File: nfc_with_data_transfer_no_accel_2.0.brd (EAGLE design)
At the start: 13.2 x 18.4 mm, 7 parts

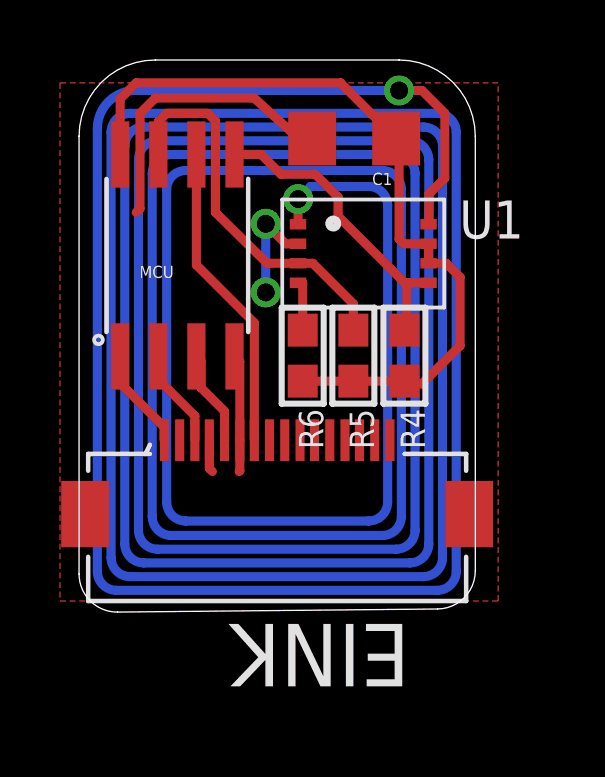
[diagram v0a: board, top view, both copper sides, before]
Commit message: fixed rst
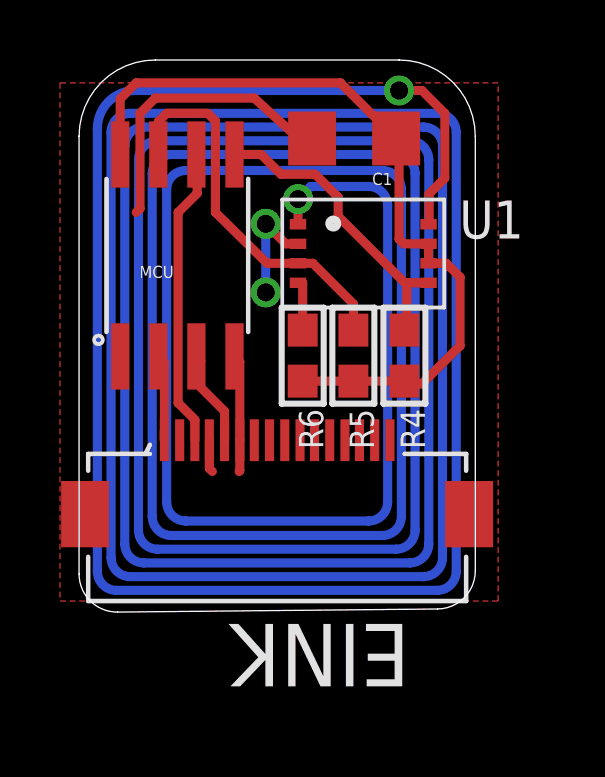
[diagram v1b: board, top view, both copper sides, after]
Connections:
- net DOT1: now also MCU.6; no longer MCU.2
- net DOT5: now also MCU.1; no longer MCU.6
- net RST: now also MCU.2; no longer MCU.1
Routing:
- net DOT5: track 10.3 -> 0.00 mm
- net DOT1: track 3.30 -> 10.0 mm
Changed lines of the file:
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@@
 <layer number="14" name="Route14" color="1" fill="6" visible="no" active="no"/>
 <layer number="15" name="Route15" color="4" fill="6" visible="no" active="no"/>
-<layer number="16" name="Bottom" color="1" fill="1" visible="yes" active="yes"/>
+<layer number="16" name="Bottom" color="1" fill="1" visible="no" active="yes"/>
 <layer number="17" name="Pads" color="2" fill="1" visible="yes" active="yes"/>
 <layer number="18" name="Vias" color="2" fill="1" visible="yes" active="yes"/>
@@
 <contactref element="EINK" pad="5"/>
 <contactref element="MCU" pad="3"/>
+<wire x1="7.5946" y1="10.4394" x2="7.747" y2="10.287" width="0.3048" layer="1"/>
 <wire x1="8.5344" y1="7.6454" x2="8.5344" y2="8.6106" width="0.3048" layer="1"/>
-<wire x1="8.5344" y1="8.6106" x2="7.747" y2="9.398" width="0.3048" layer="1"/>
-<wire x1="7.747" y1="9.398" x2="7.747" y2="10.287" width="0.3048" layer="1"/>
-<wire x1="7.747" y1="10.287" x2="7.5946" y2="10.4394" width="0.3048" layer="1"/>
+<wire x1="8.5344" y1="8.6106" x2="7.62" y2="9.525" width="0.3048" layer="1"/>
+<wire x1="7.62" y1="9.525" x2="7.62" y2="10.414" width="0.3048" layer="1"/>
+<wire x1="7.62" y1="10.414" x2="7.5946" y2="10.4394" width="0.3048" layer="1"/>
 </signal>
 <signal name="DOT1">
 <contactref element="EINK" pad="3"/>
-<contactref element="MCU" pad="2"/>
-<wire x1="7.5438" y1="7.6454" x2="7.5438" y2="8.4582" width="0.3048" layer="1"/>
-<wire x1="7.5438" y1="8.4582" x2="6.35" y2="9.652" width="0.3048" layer="1"/>
-<wire x1="6.35" y1="9.652" x2="6.35" y2="10.414" width="0.3048" layer="1"/>
-<wire x1="6.35" y1="10.414" x2="6.3246" y2="10.4394" width="0.3048" layer="1"/>
+<contactref element="MCU" pad="6"/>
+<wire x1="7.5438" y1="7.6454" x2="7.5438" y2="8.3312" width="0.3048" layer="1"/>
+<wire x1="7.5438" y1="8.3312" x2="6.985" y2="8.89" width="0.3048" layer="1"/>
+<wire x1="6.985" y1="8.89" x2="6.985" y2="15.24" width="0.3048" layer="1"/>
+<wire x1="6.985" y1="15.24" x2="7.62" y2="15.875" width="0.3048" layer="1"/>
+<wire x1="7.62" y1="15.875" x2="7.62" y2="17.145" width="0.3048" layer="1"/>
+<wire x1="7.62" y1="17.145" x2="7.5946" y2="17.1704" width="0.3048" layer="1"/>
 </signal>
 <signal name="RST">
 <contactref element="EINK" pad="1"/>
-<contactref element="MCU" pad="1"/>
 <wire x1="6.5278" y1="7.9502" x2="6.5278" y2="7.6454" width="0.3048" layer="1"/>
-<wire x1="6.5278" y1="7.6454" x2="6.5278" y2="8.0772" width="0.3048" layer="1"/>
 <wire x1="5.08" y1="9.525" x2="5.08" y2="10.414" width="0.3048" layer="1"/>
-<wire x1="5.08" y1="10.414" x2="5.0546" y2="10.4394" width="0.3048" layer="1"/>
-<wire x1="6.5278" y1="7.6454" x2="6.5278" y2="8.0772" width="0.3048" layer="1"/>
-<wire x1="6.5278" y1="8.0772" x2="5.08" y2="9.525" width="0.3048" layer="1"/>
+<contactref element="MCU" pad="2"/>
+<wire x1="6.5278" y1="7.6454" x2="6.5278" y2="10.2362" width="0.3048" layer="1"/>
+<wire x1="6.5278" y1="10.2362" x2="6.3246" y2="10.4394" width="0.3048" layer="1"/>
+<wire x1="6.3246" y1="10.4394" x2="5.08" y2="10.414" width="0" layer="19" extent="1-1"/>
 </signal>
 <signal name="2.8V">
@@
 <signal name="DOT5">
 <contactref element="EINK" pad="7"/>
-<contactref element="MCU" pad="6"/>
-<wire x1="9.525" y1="11.557" x2="9.525" y2="7.6454" width="0.3048" layer="1"/>
-<wire x1="7.5946" y1="17.1704" x2="7.5946" y2="13.4874" width="0.3048" layer="1"/>
-<wire x1="7.5946" y1="13.4874" x2="9.525" y2="11.557" width="0.3048" layer="1"/>
+<contactref element="MCU" pad="1"/>
+<wire x1="5.0546" y1="10.4394" x2="9.525" y2="7.6454" width="0" layer="19" extent="1-1"/>
 </signal>
 </signals>
